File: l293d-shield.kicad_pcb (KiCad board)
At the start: 2 copper layers, 53.3 x 43.2 mm, 4 parts, among them J1 CONN_01X04, J2 CONN_01X02, U1 l293d

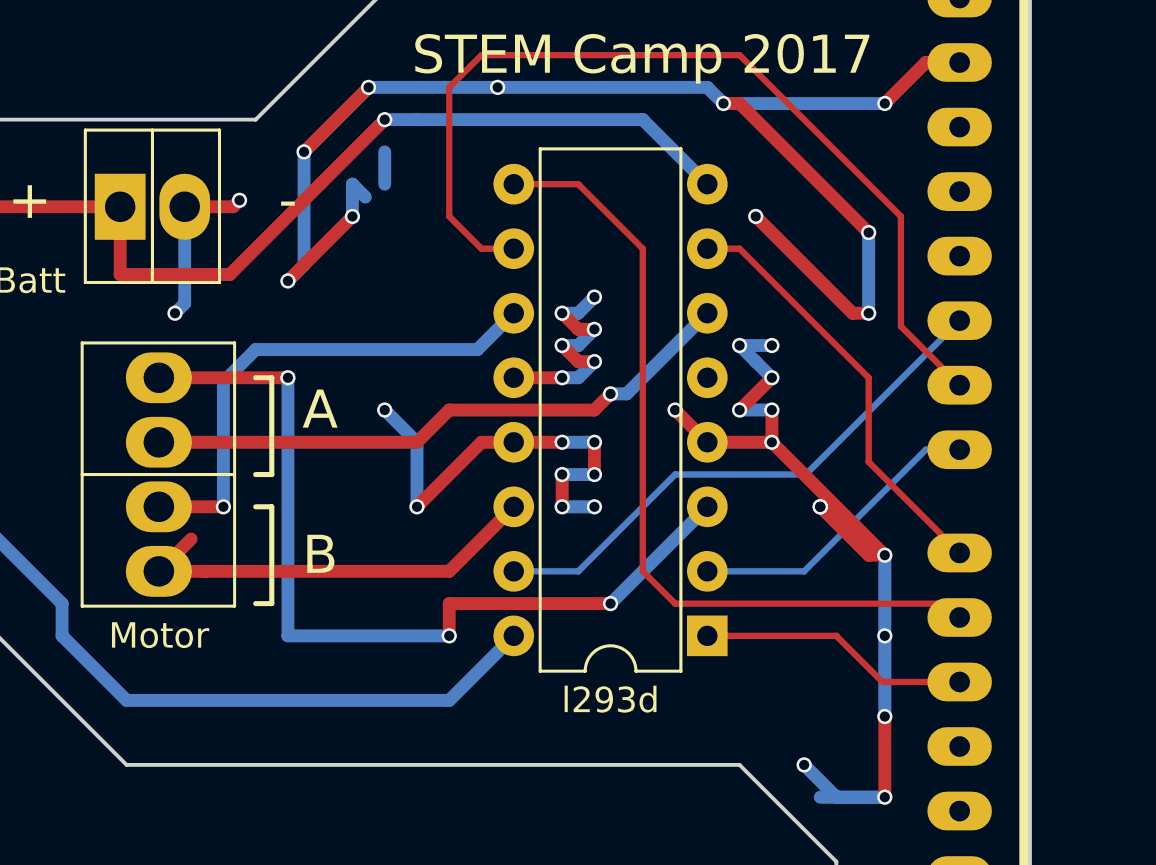
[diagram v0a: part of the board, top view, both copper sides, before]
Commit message: fix stray trace
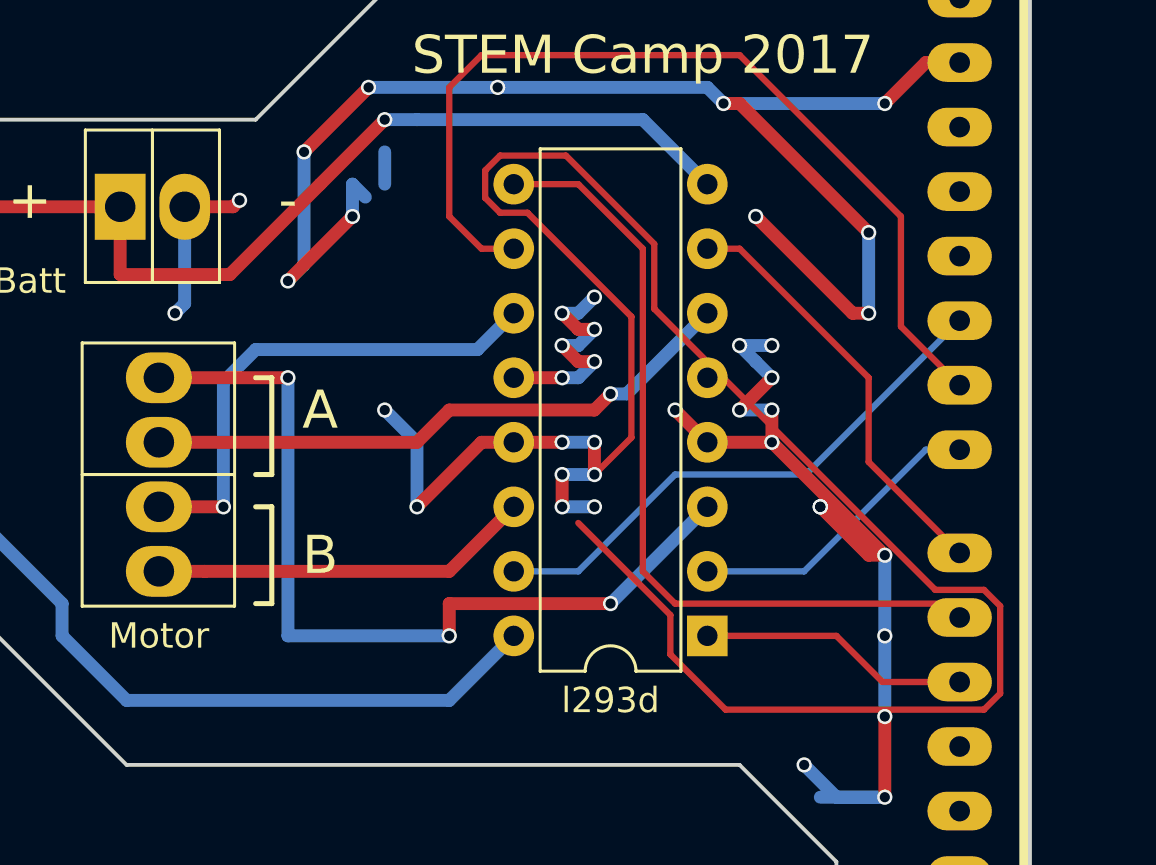
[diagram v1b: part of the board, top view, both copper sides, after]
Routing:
- net GND: track 152.5 -> 221.7 mm
- net /OUT_4: track 16.8 -> 15.0 mm
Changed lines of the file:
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@@
   (general
     (links 20)
-    (no_connects 1)
+    (no_connects 0)
     (area 154.2614 49.295529 213.433 122.856601)
     (thickness 1.6)
     (drawings 26)
-    (tracks 193)
+    (tracks 211)
     (zones 0)
     (modules 4)
@@
   )
   (setup
-    (last_trace_width 0.508)
+    (last_trace_width 0.25)
     (user_trace_width 0.508)
     (trace_clearance 0.2)
@@
     (visible_elements FFFFFF7F)
     (pcbplotparams
-      (layerselection 0x00030_80000001)
-      (usegerberextensions false)
+      (layerselection 0x010f0_80000001)
+      (usegerberextensions true)
       (excludeedgelayer true)
       (linewidth 0.100000)
@@
       (plotinvisibletext false)
       (padsonsilk false)
-      (subtractmaskfromsilk false)
+      (subtractmaskfromsilk true)
       (outputformat 1)
       (mirror false)
-      (drillshape 1)
+      (drillshape 0)
       (scaleselection 1)
-      (outputdirectory ""))
+      (outputdirectory out/))
   )
   (net 0 "")
@@
   (segment (start 192.405 93.345) (end 191.77 93.345) (width 0.508) (layer B.Cu) (net 19))
   (segment (start 195.58 90.17) (end 192.405 93.345) (width 0.508) (layer B.Cu) (net 19))
-  (segment (start 173.99 100.33) (end 175.26 99.06) (width 0.508) (layer F.Cu) (net 20))
   (segment (start 187.96 97.79) (end 185.42 100.33) (width 0.508) (layer F.Cu) (net 20))
   (segment (start 173.99 100.33) (end 175.798 100.33) (width 0.508) (layer F.Cu) (net 20))
@@
   (segment (start 160.5661 91.9861) (end 170.18 101.6) (width 0.508) (layer B.Cu) (net 28))
   (segment (start 157.2514 91.9861) (end 160.5661 91.9861) (width 0.508) (layer B.Cu) (net 28))
+  (segment (start 191.135 96.52) (end 192.58999 95.06501) (width 0.25) (layer F.Cu) (net 29))
+  (segment (start 193.49001 89.995954) (end 204.553146 101.05909) (width 0.25) (layer F.Cu) (net 29))
+  (segment (start 204.553146 101.05909) (end 206.469654 101.05909) (width 0.25) (layer F.Cu) (net 29))
+  (segment (start 187.419999 83.964999) (end 190.011409 83.964999) (width 0.25) (layer F.Cu) (net 29))
+  (segment (start 192.58999 95.06501) (end 192.58999 90.30499) (width 0.25) (layer F.Cu) (net 29))
+  (segment (start 192.58999 90.30499) (end 188.500001 86.215001) (width 0.25) (layer F.Cu) (net 29))
+  (segment (start 188.500001 86.215001) (end 187.419999 86.215001) (width 0.25) (layer F.Cu) (net 29))
+  (segment (start 186.834999 85.630001) (end 186.834999 84.549999) (width 0.25) (layer F.Cu) (net 29))
+  (segment (start 187.419999 86.215001) (end 186.834999 85.630001) (width 0.25) (layer F.Cu) (net 29))
+  (segment (start 186.834999 84.549999) (end 187.419999 83.964999) (width 0.25) (layer F.Cu) (net 29))
+  (segment (start 190.011409 83.964999) (end 193.49001 87.4436) (width 0.25) (layer F.Cu) (net 29))
+  (segment (start 193.49001 87.4436) (end 193.49001 89.995954) (width 0.25) (layer F.Cu) (net 29))
+  (segment (start 206.469654 101.05909) (end 207.10641 101.695846) (width 0.25) (layer F.Cu) (net 29))
+  (segment (start 207.10641 101.695846) (end 207.10641 105.136354) (width 0.25) (layer F.Cu) (net 29))
+  (segment (start 207.10641 105.136354) (end 206.469654 105.77311) (width 0.25) (layer F.Cu) (net 29))
+  (segment (start 194.1236 102.05001) (end 190.5 98.42641) (width 0.25) (layer F.Cu) (net 29))
+  (segment (start 206.469654 105.77311) (end 196.298108 105.77311) (width 0.25) (layer F.Cu) (net 29))
+  (segment (start 196.298108 105.77311) (end 194.1236 103.598602) (width 0.25) (layer F.Cu) (net 29))
+  (segment (start 194.1236 103.598602) (end 194.1236 102.05001) (width 0.25) (layer F.Cu) (net 29))
   (segment (start 181.61 86.36) (end 181.61 85.09) (width 0.508) (layer B.Cu) (net 29))
   (segment (start 181.61 85.09) (end 182.11799 85.59799) (width 0.508) (layer B.Cu) (net 29))
